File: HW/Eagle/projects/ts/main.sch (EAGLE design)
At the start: 45 parts, among them IC1 4050D, Q1 20 MHz, T1 IRFZ24N, T2 IRFZ24N, U1 ATMEGA328P-PU, U2 LM2576T, U3 HT7533, U4 LM75

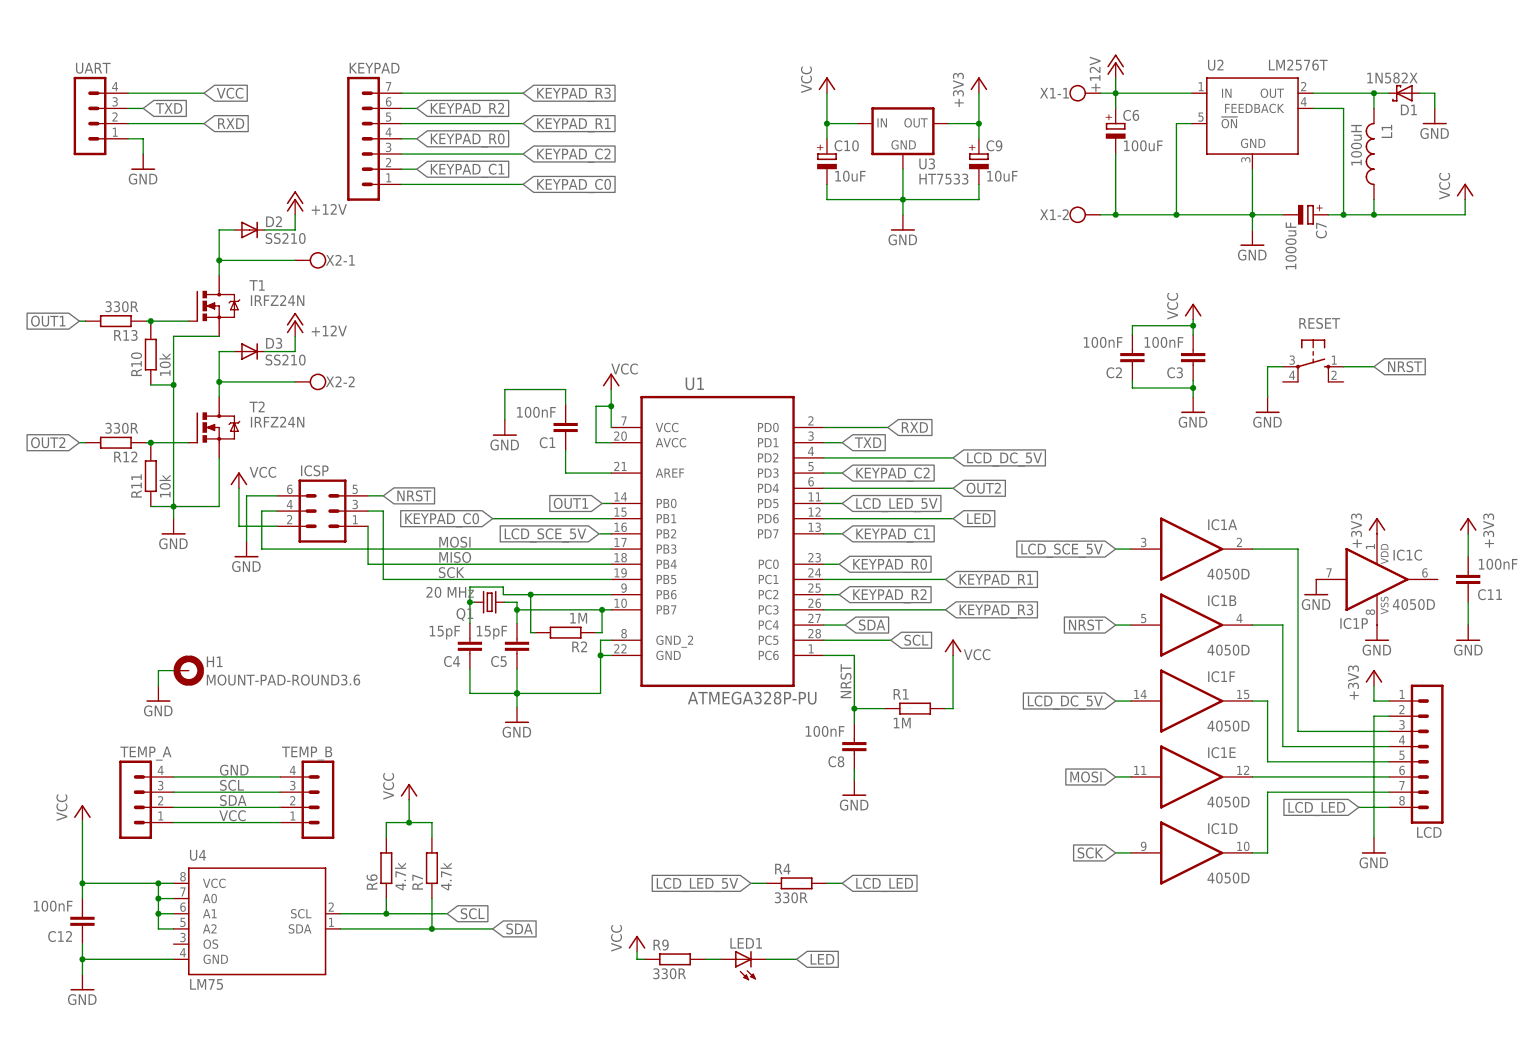
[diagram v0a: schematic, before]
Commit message: [HW] Organized schematics
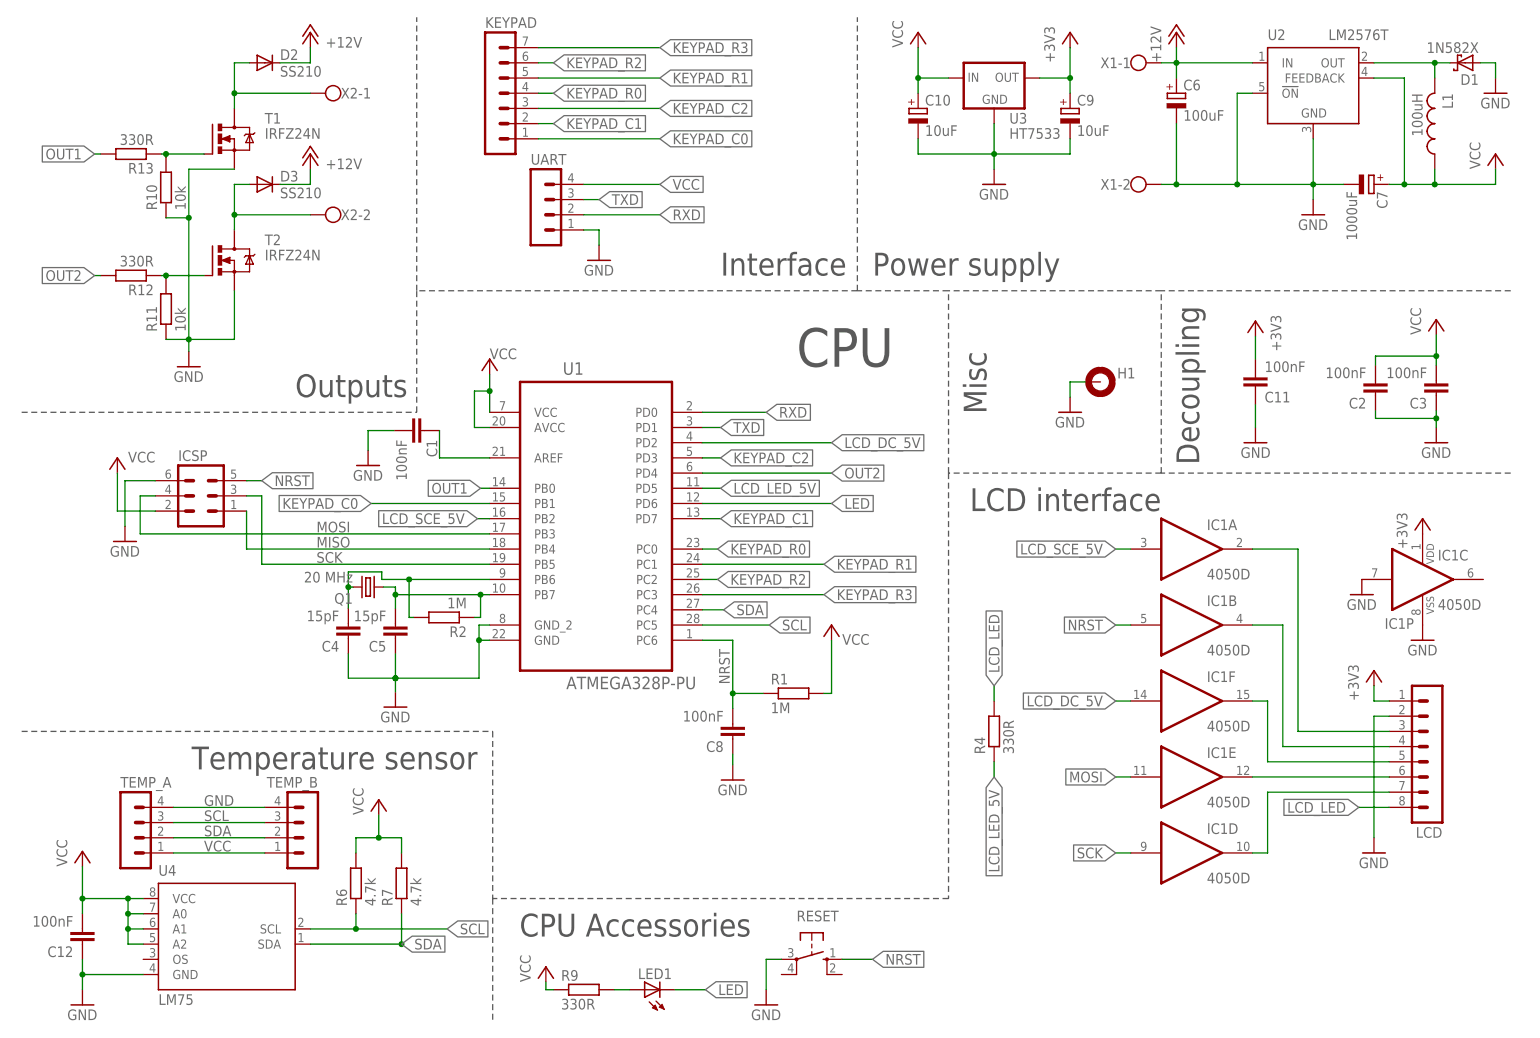
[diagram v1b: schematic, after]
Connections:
- net AREF renamed N$1
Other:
- note added: "CPU"
- note added: "CPU Accessories"
- note added: "Decoupling"
- note added: "Interface"
- note added: "LCD interface"
- note added: "Misc"
- note added: "Outputs"
- note added: "Power supply"
- note added: "Temperature sensor"
- moved on the sheet: C1, C10, C11, C12, C2, C3, C4, C5, C6, C7, C8, C9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
